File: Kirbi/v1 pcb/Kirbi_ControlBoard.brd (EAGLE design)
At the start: 66 x 56 mm, 66 parts, among them U1 PCA9306_LSSOP, U2 TEENSY_3.6_DIL, U5 LM393-8-SOIC, U6 AP2114H-1.8TRG1, U7 AP2114H-3.3TRG1

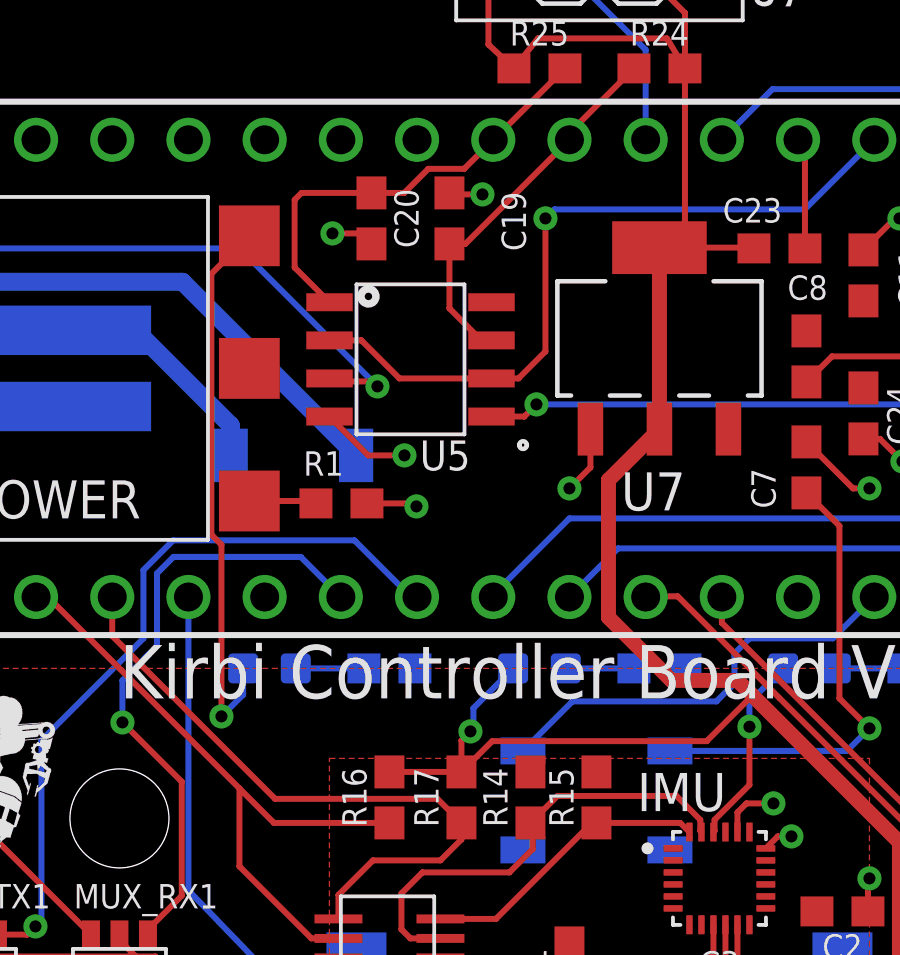
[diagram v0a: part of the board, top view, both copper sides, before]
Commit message: Added Pull-up Resistors/Moved MUXs
Added Pull-up Resistors (1k OHM to RX line)
Added 6.2 OHM to 1.8 V LED
Moved MUXs and rerouted
Fixed SIlkscreen
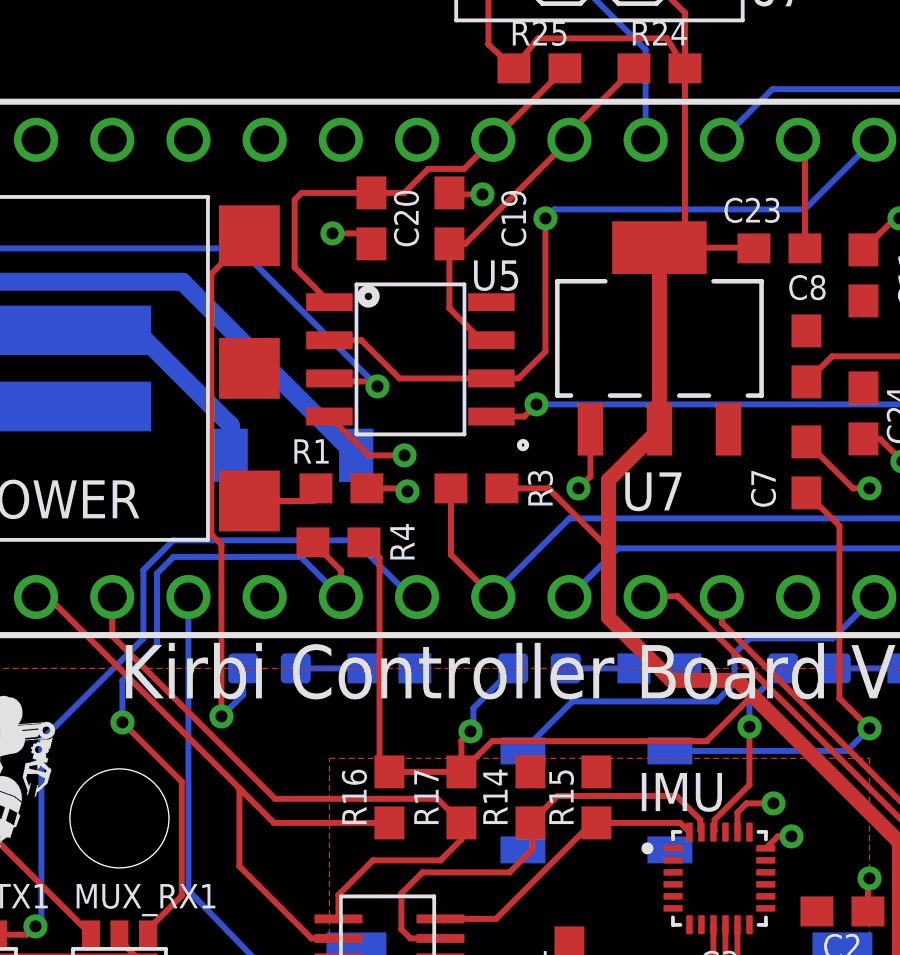
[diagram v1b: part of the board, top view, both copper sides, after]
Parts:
- added R3, R4: 1k, SparkFun-Resistors:0603
- moved R1 0.50 mm to (10.4, 34.0)
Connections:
- net +3.3V: now also R3.2, R4.2
- net TRX1: now also R4.1
- net TRX2: now also R3.1
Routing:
- net +3.3V: track 156.3 -> 168.7 mm
- net TRX2: track 37.3 -> 41.5 mm
- net TRX1: track 20.7 -> 22.9 mm
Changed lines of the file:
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@@
 </element>
 <element name="U5" library="Gucci_ControlBoard" package="8-SOIC" value="LM393-8-SOIC" x="12.7" y="38.3" smashed="yes">
-<attribute name="NAME" x="14.7" y="35.6" size="1" layer="25" font="vector" rot="R180"/>
+<attribute name="NAME" x="16.4" y="41.6" size="1" layer="25" font="vector" rot="R180"/>
 <attribute name="VALUE" x="10.7" y="34.5" size="1" layer="27"/>
 </element>
@@
 </element>
 <element name="C19" library="SparkFun-Capacitors" library_urn="urn:adsk.eagle:library:510" package="0603" package3d_urn="urn:adsk.eagle:package:37414/1" value="15pF" x="14" y="43" smashed="yes" rot="R90">
-<attribute name="NAME" x="15.738" y="42.9" size="0.8128" layer="25" font="vector" ratio="20" rot="R270" align="bottom-center"/>
+<attribute name="NAME" x="15.738" y="43" size="0.8128" layer="25" font="vector" ratio="20" rot="R270" align="bottom-center"/>
 <attribute name="PROD_ID" value="CAP-00810" x="14" y="43" size="1.778" layer="27" rot="R90" display="off"/>
 <attribute name="VALUE" x="14.762" y="43" size="0.6096" layer="27" font="vector" ratio="20" rot="R90" align="top-center"/>
@@
 <attribute name="NAME" x="22.3925" y="22.0125" size="0.8128" layer="26" font="vector" ratio="10" rot="MR90"/>
 </element>
-<element name="R1" library="SparkFun-Resistors" library_urn="urn:adsk.eagle:library:532" package="0603" package3d_urn="urn:adsk.eagle:package:39650/1" value="100" x="10.4" y="33.5" smashed="yes" rot="R180">
-<attribute name="NAME" x="9.8" y="35.238" size="0.8128" layer="25" font="vector" ratio="20" rot="R180" align="bottom-center"/>
-<attribute name="PROD_ID" value="RES-12438" x="10.4" y="33.5" size="1.778" layer="27" rot="R180" display="off"/>
-<attribute name="VALUE" value="100" x="10.4" y="34.262" size="0.6096" layer="27" font="vector" ratio="20" rot="R180" align="top-center"/>
+<element name="R1" library="SparkFun-Resistors" library_urn="urn:adsk.eagle:library:532" package="0603" package3d_urn="urn:adsk.eagle:package:39650/1" value="100" x="10.4" y="34" smashed="yes" rot="R180">
+<attribute name="NAME" x="9.4" y="35.638" size="0.8128" layer="25" font="vector" ratio="20" rot="R180" align="bottom-center"/>
+<attribute name="PROD_ID" value="RES-12438" x="10.4" y="34" size="1.778" layer="27" rot="R180" display="off"/>
+<attribute name="VALUE" value="100" x="10.4" y="34.762" size="0.6096" layer="27" font="vector" ratio="20" rot="R180" align="top-center"/>
 </element>
 <element name="MUX_TX1" library="Kirbi_ControlBoard" package="MUX_74LVC1G157GV" value="MUX_74LVC1G157GV" x="-2" y="18" smashed="yes">
@@
 </element>
 <element name="F1" library="Kirbi_ControlBoard" package="BEL_FUSE_C1F_3.5" value="3.5" x="8.8" y="35.1" smashed="yes" rot="MR180">
-<attribute name="NAME" x="12.852" y="36.095" size="1.778" layer="26" font="vector" rot="MR180"/>
+<attribute name="NAME" x="5.752" y="37.595" size="1.016" layer="26" font="vector" rot="MR180"/>
 <attribute name="VALUE" x="5.879" y="38.656" size="1.778" layer="28" font="vector" rot="MR180"/>
 </element>
 <element name="R2" library="Kirbi_ControlBoard" package="0603" package3d_urn="urn:adsk.eagle:package:39650/1" value="6.2" x="30" y="28" smashed="yes" rot="MR180">
-<attribute name="NAME" x="30" y="27.238" size="0.6096" layer="26" font="vector" ratio="20" rot="MR180" align="bottom-center"/>
+<attribute name="NAME" x="30" y="27.238" size="0.8128" layer="26" font="vector" ratio="20" rot="MR180" align="bottom-center"/>
 <attribute name="PROD_ID" value="P6.2GCT-ND" x="30" y="28" size="1.778" layer="28" rot="MR180" display="off"/>
 <attribute name="VALUE" x="30" y="28.762" size="0.6096" layer="28" font="vector" ratio="20" rot="MR180" align="top-center"/>
+</element>
+<element name="R3" library="SparkFun-Resistors" library_urn="urn:adsk.eagle:library:532" package="0603" package3d_urn="urn:adsk.eagle:package:39650/1" value="1k" x="14.9" y="34" smashed="yes">
+<attribute name="NAME" x="17.438" y="34" size="0.8128" layer="25" font="vector" ratio="20" rot="R90" align="bottom-center"/>
+<attribute name="PROD_ID" value="RES-07856" x="14.9" y="34" size="1.778" layer="27" display="off"/>
+<attribute name="VALUE" x="14.9" y="33.238" size="0.6096" layer="27" font="vector" ratio="20" align="top-center"/>
+</element>
+<element name="R4" library="SparkFun-Resistors" library_urn="urn:adsk.eagle:library:532" package="0603" package3d_urn="urn:adsk.eagle:package:39650/1" value="1k" x="10.3" y="32.2" smashed="yes">
+<attribute name="NAME" x="12.838" y="32.2" size="0.8128" layer="25" font="vector" ratio="20" rot="R90" align="bottom-center"/>
+<attribute name="PROD_ID" value="RES-07856" x="10.3" y="32.2" size="1.778" layer="27" display="off"/>
+<attribute name="VALUE" x="10.3" y="31.438" size="0.6096" layer="27" font="vector" ratio="20" align="top-center"/>
 </element>
 </elements>
@@
 <wire x1="30.625" y1="3.375" x2="30.8" y2="3.2" width="0.2" layer="1"/>
 <via x="30.8" y="3.2" extent="1-16" drill="0.4"/>
-<wire x1="18.7" y1="35.975" x2="18.7" y2="34.7" width="0.2" layer="1"/>
-<wire x1="18.7" y1="34.7" x2="18" y2="34" width="0.2" layer="1"/>
-<via x="18" y="34" extent="1-16" drill="0.4"/>
+<wire x1="18.7" y1="35.975" x2="18.7" y2="34.4" width="0.2" layer="1"/>
+<wire x1="18.7" y1="34.4" x2="18.3" y2="34" width="0.2" layer="1"/>
+<via x="18.3" y="34" extent="1-16" drill="0.4"/>
 <contactref element="DIST_2" pad="P$3"/>
 <contactref element="DIST_5" pad="P$3"/>
@@
 <via x="10.1" y="42.5" extent="1-16" drill="0.4"/>
 <contactref element="POWER_CONN" pad="P$2"/>
-<wire x1="11.25" y1="33.5" x2="12.8" y2="33.5" width="0.2" layer="1"/>
-<wire x1="12.8" y1="33.5" x2="12.9" y2="33.4" width="0.2" layer="1"/>
-<via x="12.9" y="33.4" extent="1-16" drill="0.4"/>
+<via x="12.6" y="33.9" extent="1-16" drill="0.4"/>
 <wire x1="23.6" y1="23.2" x2="23.9" y2="23.5" width="0.2" layer="1"/>
 <wire x1="23.9" y1="23.5" x2="24.8" y2="23.5" width="0.2" layer="1"/>
@@
 <contactref element="ESC" pad="P$3"/>
 <contactref element="R2" pad="2"/>
+<wire x1="11.25" y1="34" x2="12.5" y2="34" width="0.2" layer="1"/>
+<wire x1="12.5" y1="34" x2="12.6" y2="33.9" width="0.2" layer="1"/>
 </signal>
 <signal name="+5V">
@@
 <wire x1="21.4" y1="27.6" x2="19.301" y2="29.699" width="0.5" layer="1"/>
 <wire x1="19.301" y1="34.276" x2="21" y2="35.975" width="0.5" layer="1"/>
-<wire x1="19.301" y1="29.699" x2="19.301" y2="34.276" width="0.5" layer="1"/>
+<wire x1="19.301" y1="29.699" x2="19.301" y2="32" width="0.5" layer="1"/>
+<wire x1="19.301" y1="32" x2="19.301" y2="34.276" width="0.5" layer="1"/>
 <wire x1="15.425" y1="25.575" x2="22.575" y2="25.575" width="0.2" layer="1"/>
 <wire x1="22.575" y1="25.575" x2="24.1" y2="27.1" width="0.2" layer="1"/>
@@
 <wire x1="16.123" y1="28" x2="14.8" y2="26.677" width="0.2" layer="16"/>
 <wire x1="14.8" y1="26.677" x2="14.8" y2="26" width="0.2" layer="16"/>
+<contactref element="R3" pad="2"/>
+<contactref element="R4" pad="2"/>
+<wire x1="15.75" y1="34" x2="17.301" y2="34" width="0.2" layer="1"/>
+<wire x1="17.301" y1="34" x2="19.301" y2="32" width="0.2" layer="1"/>
+<wire x1="11.15" y1="32.2" x2="11.669" y2="31.681" width="0.2" layer="1"/>
+<wire x1="11.669" y1="31.681" x2="11.669" y2="24.881" width="0.2" layer="1"/>
+<wire x1="11.669" y1="24.881" x2="12" y2="24.55" width="0.2" layer="1"/>
 </signal>
 <signal name="LINE_LF">
@@
 <contactref element="R1" pad="2"/>
 <wire x1="9.47" y1="33.58" x2="7.33" y2="33.58" width="0.2" layer="1"/>
-<wire x1="9.55" y1="33.5" x2="9.47" y2="33.58" width="0.2" layer="1"/>
+<wire x1="9.55" y1="34" x2="9.47" y2="33.58" width="0.2" layer="1"/>
 </signal>
 <signal name="MISO">
@@
 <wire x1="3.1" y1="26.2" x2="5.077" y2="24.223" width="0.2" layer="1"/>
 <wire x1="5.077" y1="24.223" x2="5.077" y2="20.42251875" width="0.2" layer="1"/>
+<contactref element="R4" pad="1"/>
+<wire x1="9.45" y1="32.2" x2="10.38" y2="31.27" width="0.2" layer="1"/>
+<wire x1="10.38" y1="31.27" x2="10.38" y2="30.38" width="0.2" layer="1"/>
 </signal>
 <signal name="TXD6">
@@
 <wire x1="37.1" y1="31.7" x2="35.8" y2="33" width="0.2" layer="16"/>
 <wire x1="35.8" y1="33" x2="18" y2="33" width="0.2" layer="16"/>
+<contactref element="R3" pad="1"/>
+<wire x1="14.05" y1="34" x2="14.05" y2="31.79" width="0.2" layer="1"/>
+<wire x1="14.05" y1="31.79" x2="15.46" y2="30.38" width="0.2" layer="1"/>
 </signal>
 <signal name="TTX1">
